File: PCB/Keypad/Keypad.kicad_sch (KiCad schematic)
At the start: 21 parts, among them J1 Keypad, J2 Shelly, U1 SP3485, U2 ESP32-PICO-MINI-02, U2 LMR16006YDDCR, U4 QR

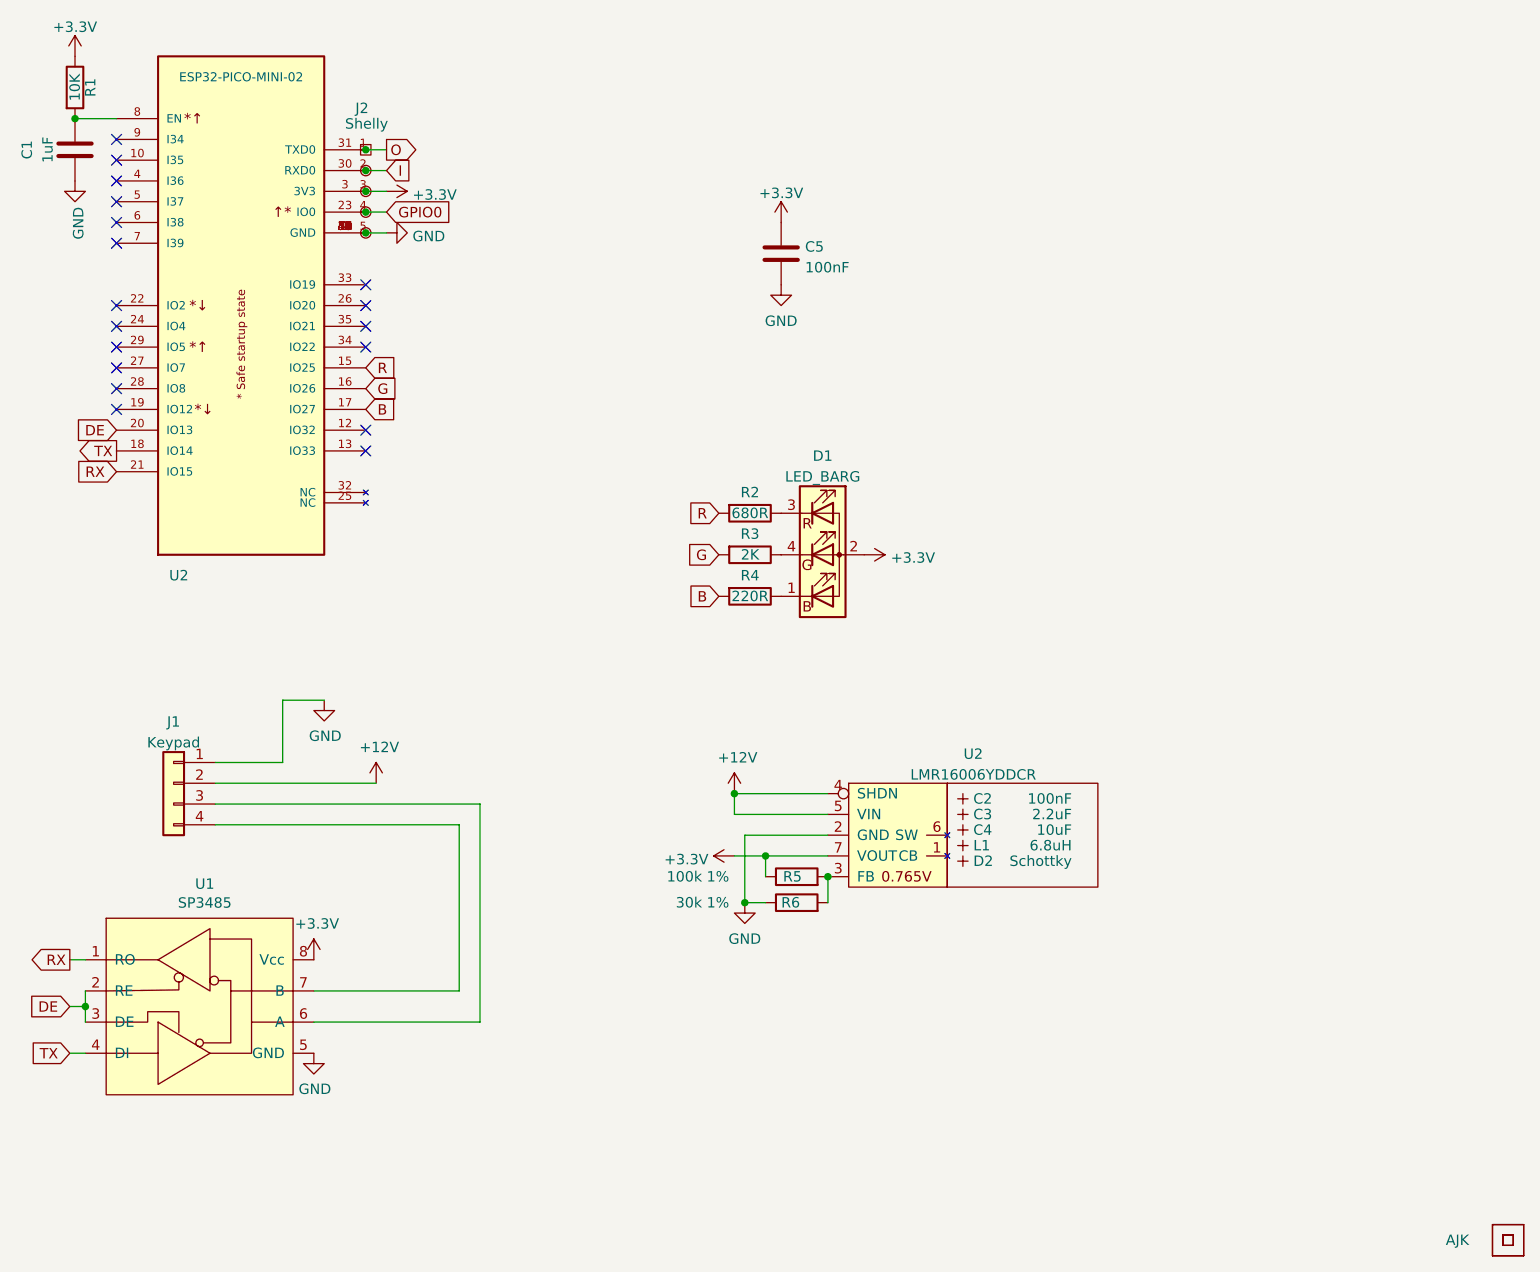
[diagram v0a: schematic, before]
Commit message: Tidy, new PSU and LED
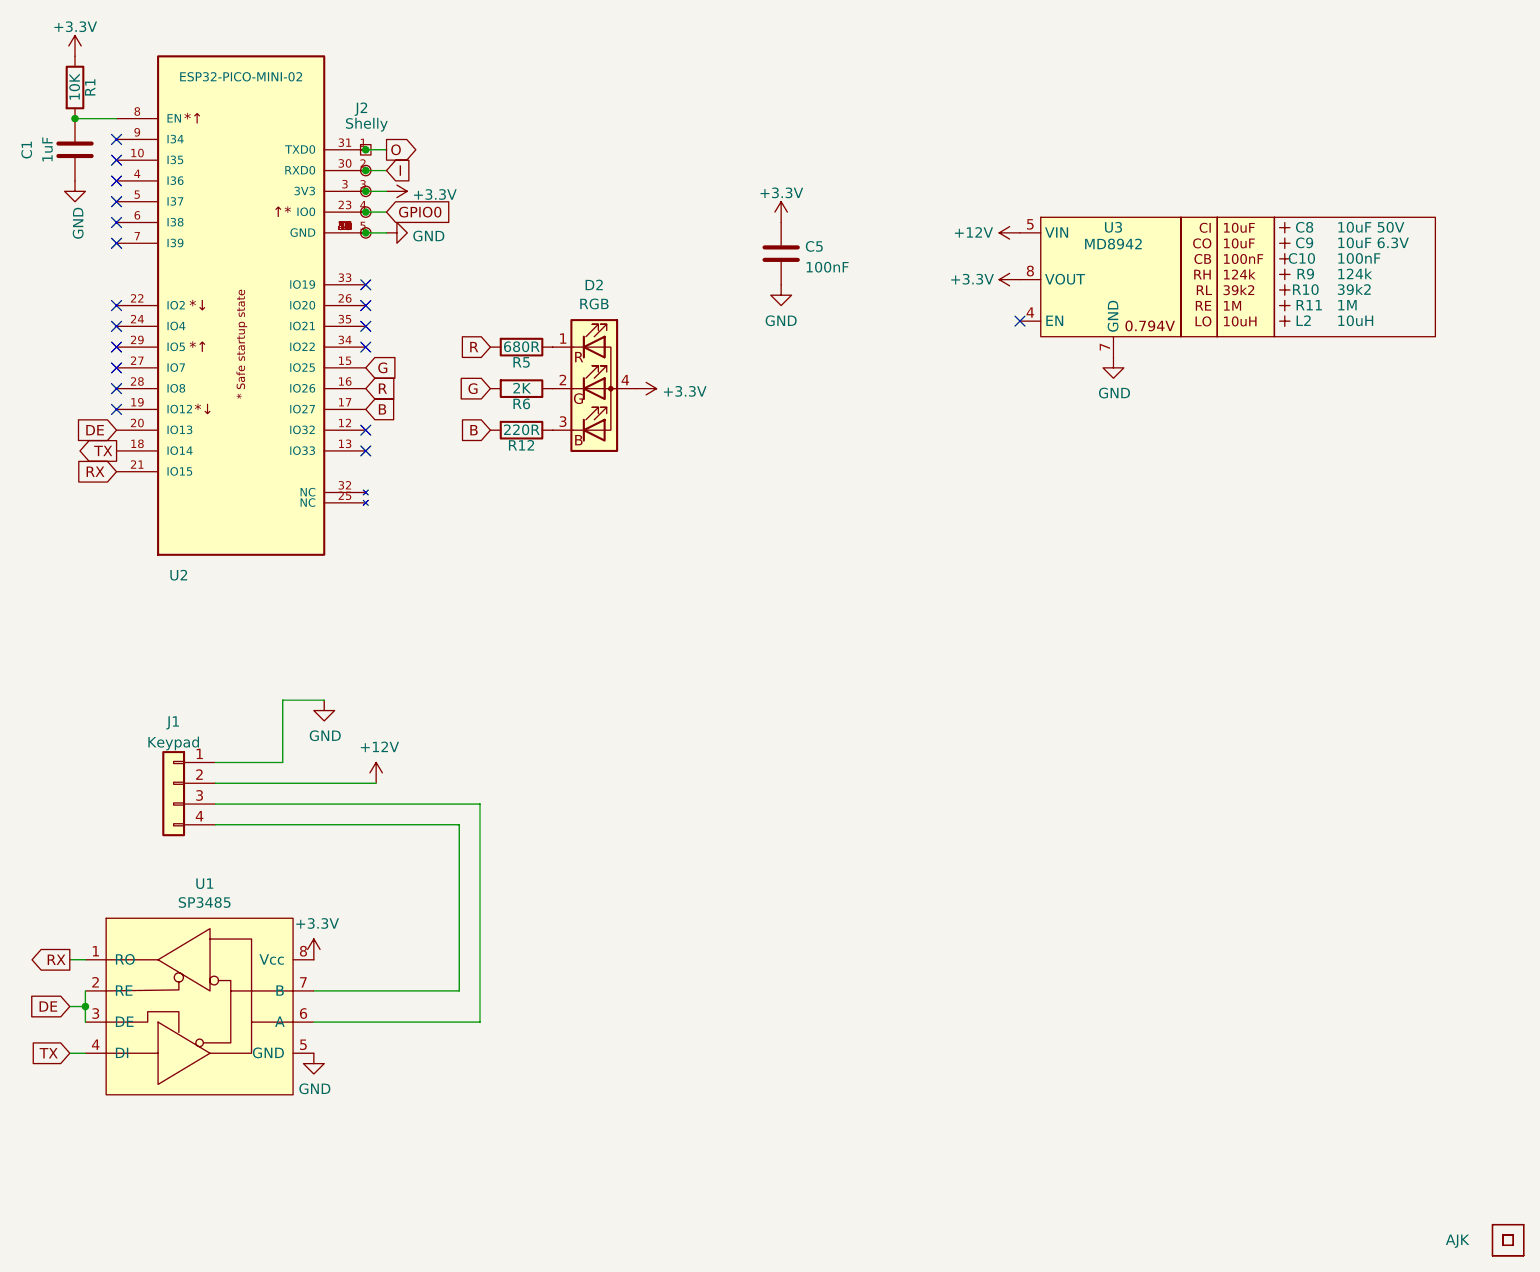
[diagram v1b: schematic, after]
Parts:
- removed C2: 100nF, RevK:C_0603_, symbol RevK:Hidden
- removed C3: 2.2uF, RevK:C_0805_, symbol RevK:Hidden
- removed C4: 10uF, RevK:C_0805_, symbol RevK:Hidden
- removed D1: LED_BARG, RevK:MHS190RGBCT, symbol Device:LED_BARG
- removed D2: Schottky, RevK:D_1206_, symbol RevK:Hidden
- removed L1: 6.8uH, RevK:L_4x4_, symbol RevK:Hidden
- removed R2: 680R, RevK:R_0603, symbol Device:R
- removed R3: 2K, RevK:R_0603, symbol Device:R
- removed R4: 220R, RevK:R_0603, symbol Device:R
- removed U2: LMR16006YDDCR, RevK:SOT-23-Thin-6-Reg, symbol RevK:LMR16006XDDCR
- added C10: 100nF, RevK:C_0603_, symbol RevK:Hidden
- added C8: 10uF 50V, RevK:C_0603_, symbol RevK:Hidden
- added C9: 10uF 6.3V, RevK:C_0603_, symbol RevK:Hidden
- added D2: RGB, RevK:LED-RGB-1.6x1.6, symbol Device:LED_RGBA
- added L2: 10uH, RevK:L_4x4_, symbol RevK:Hidden
- added R10: 39k2, RevK:R_0402_, symbol RevK:Hidden
- added R11: 1M, RevK:R_0402_, symbol RevK:Hidden
- added R12: 220R, RevK:R_0402, symbol Device:R
- added R9: 124k, RevK:R_0402_, symbol RevK:Hidden
- added U3: MD8942, RevK:SOT-23-6-MD8942, symbol RevK:MD89420-RegBlock
- C1, C5: footprint RevK:C_0603 -> RevK:C_0402
- R1: footprint RevK:R_0603 -> RevK:R_0402
- R5: value 100k 1% -> 680R; footprint RevK:R_0603 -> RevK:R_0402; LCSC Part # C14675 -> (none)
- R6: value 30k 1% -> 2K; footprint RevK:R_0603 -> RevK:R_0402; LCSC Part # C100001 -> (none)
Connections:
- net +12V: now also U3.5 (VIN)
- net +3V3: now also D2.4 (A), U3.8 (VOUT); no longer R5.1
- net B: now also R12.2
- net G: now also R6.2, U2.15 (IO25); no longer U2.16 (IO26)
- net GND: now also U3.2 (GND), U3.7 (GND); no longer R6.1
- net R: now also R5.2, U2.16 (IO26); no longer U2.15 (IO25)
- new net: D2.2 (GK), R6.1
- new net: D2.3 (BK), R12.1
- new net: D2.1 (RK), R5.1
- no-connect marks 18 -> 19
